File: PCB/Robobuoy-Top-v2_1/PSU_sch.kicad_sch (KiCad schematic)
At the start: 59 parts, among them J201 CHRG/DATA, Q117 MMBT3904, Q201 MMBT3904, Q203 AO3400A, Q204 AO3401A, SW201 On/Off, U201 LM1117S-3.3, U202 LMR16020PDDA

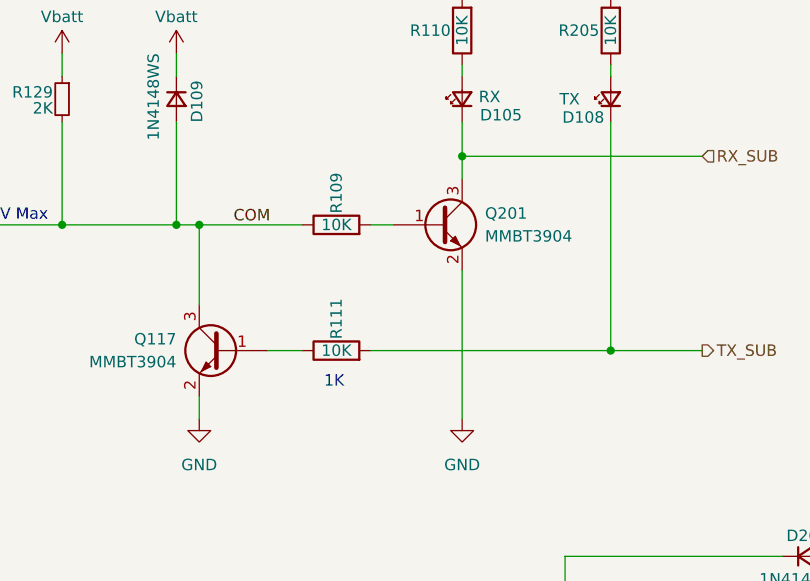
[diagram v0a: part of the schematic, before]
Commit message: Many changes
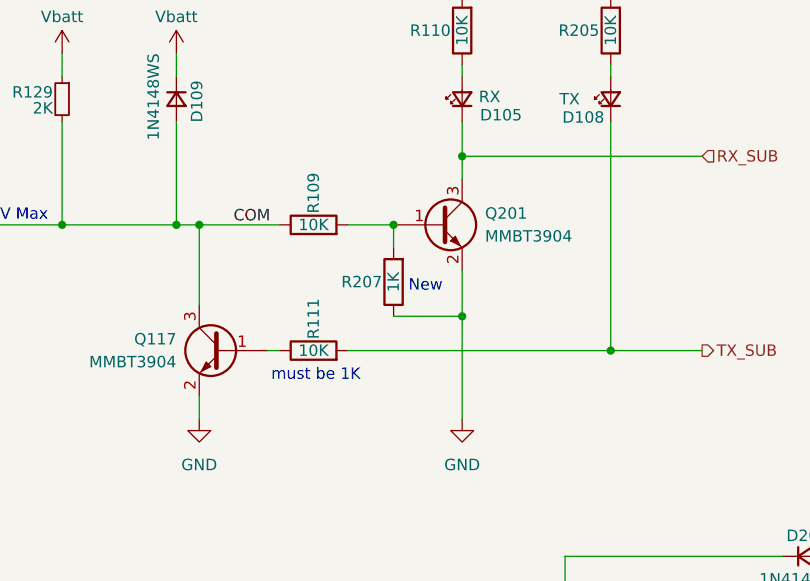
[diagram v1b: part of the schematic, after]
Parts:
- added R207: 1K, A_Device:R_0603, symbol Device:R
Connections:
- net GND: now also R207.1
- net at Q201.1 (B), R109.2: now also R207.2
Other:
- note added: "New"
- note added: "must be 1K"
- note removed: "1K"
- moved on the sheet: R109, R111
